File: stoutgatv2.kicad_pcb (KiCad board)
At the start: 2 copper layers, 345.7 x 99.5 mm, 191 parts, among them SW1 ESC, SW10 9, SW11 0, SW12 Rotary_Encoder_Switch, SW13 -, SW14 +, SW15 BKSPC, SW16 TILDE, SW17 TAB, SW18 Rotary_Encoder_Switch, SW19 Q, SW2 1, SW20 W, SW21 E, SW22 R, SW23 T, SW24 Y, SW25 U, SW26 I, SW27 O, SW28 P, SW29 [, SW3 2, SW30 ], SW31 ISO-ENTER, SW32 DEL, SW33 CAPS, SW34 A, SW35 S, SW36 D, SW37 F, SW38 G, SW39 H, SW4 3, SW40 J, SW41 K, SW42 L, SW43 ;, SW44 ', SW45 \, SW46 ANSISHIFT, SW47 CTRL-w, SW48 PGUP, SW49 SHIFT, SW5 4, SW50 <, SW51 Z, SW52 X, SW53 C, SW54 V, SW55 B, SW56 N, SW57 M, SW58 ,, SW59 ., SW6 5, SW60 /, SW61 SUPER-w, SW62 SHIFT, SW63 ^, SW64 PGDN, SW65 CTRL, SW66 SUPER, SW67 ALT, SW68 ALT-w, SW69 CTRL-w, SW7 6, SW70 ANSI-ENTER, SW71 SPACE, SW72 ANSI-|, SW73 CAPS, SW74 SPACE, SW75 ALT, SW76 FN, SW77 CTRL, SW78 <-, SW79 DN, SW8 7, SW80 ->, SW81 Rotary_Encoder_Switch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

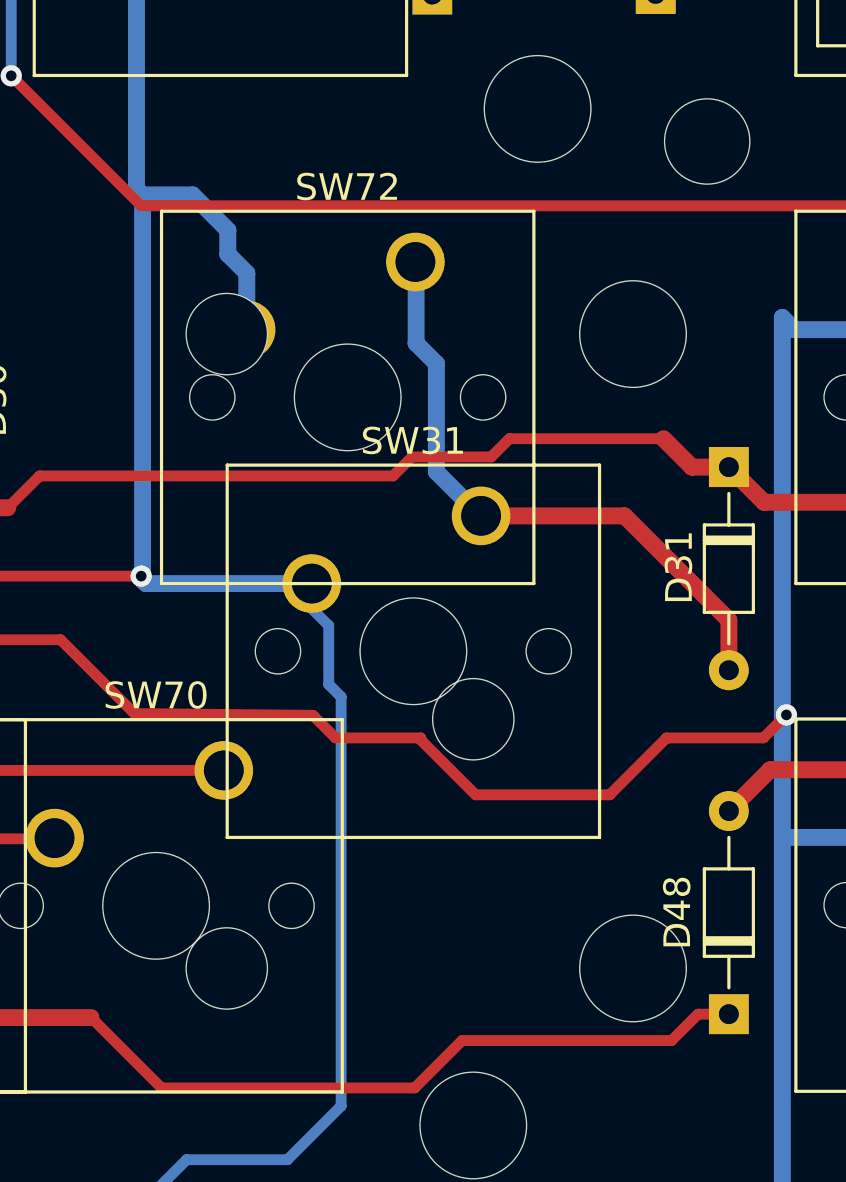
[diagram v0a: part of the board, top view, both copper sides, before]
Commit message: JLC tweaks
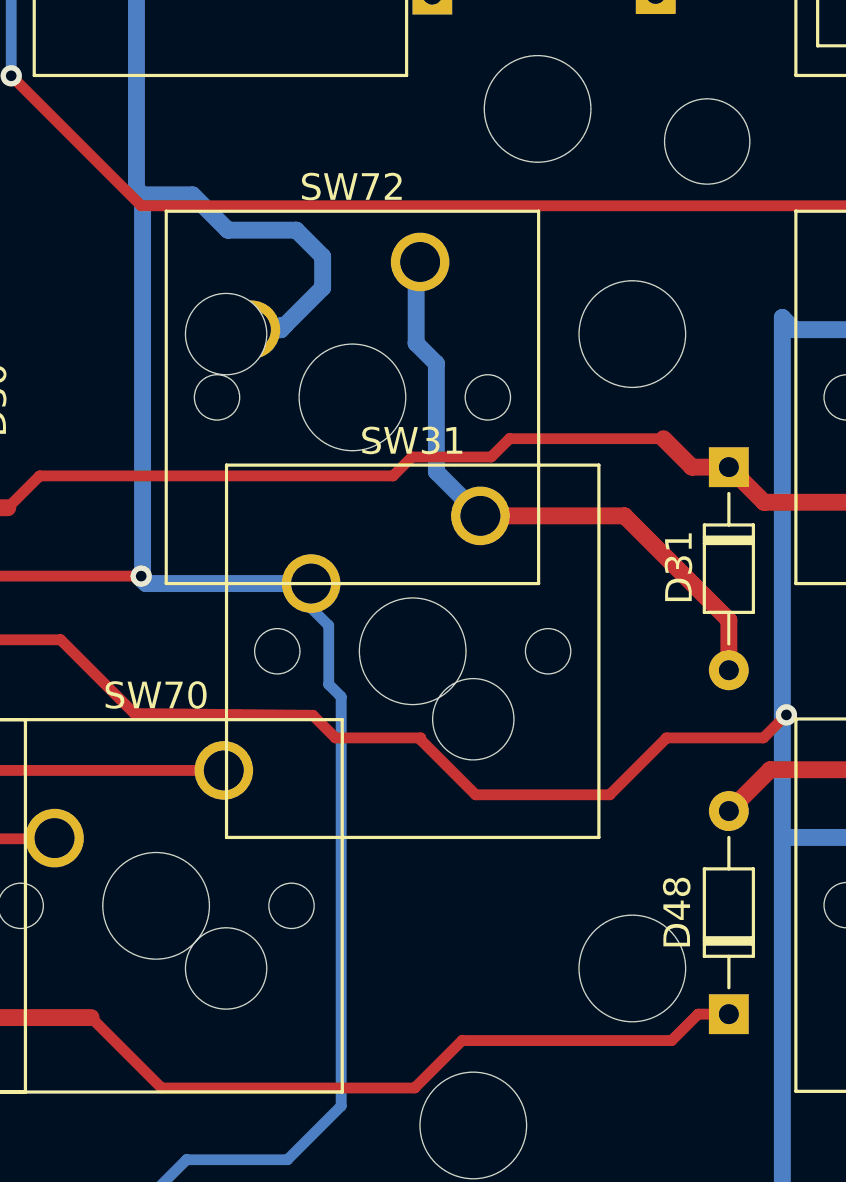
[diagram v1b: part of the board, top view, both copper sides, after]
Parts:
- moved SW72 0.18 mm to (354.5, 109.5)
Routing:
- net col13: track 422.9 -> 427.6 mm
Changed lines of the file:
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@@
     (thickness 1.6)
     (drawings 10)
-    (tracks 1026)
+    (tracks 1031)
     (zones 0)
     (modules 191)
@@
   )
   (setup
-    (last_trace_width 0.4064)
+    (last_trace_width 0.635)
     (user_trace_width 0.4064)
     (user_trace_width 0.635)
@@
     (visible_elements FFFDFF7F)
     (pcbplotparams
-      (layerselection 0x010fc_ffffffff)
+      (layerselection 0x01000_7ffffffe)
       (usegerberextensions false)
       (usegerberattributes false)
@@
       (psnegative false)
       (psa4output false)
-      (plotreference true)
-      (plotvalue true)
+      (plotreference false)
+      (plotvalue false)
       (plotinvisibletext false)
       (padsonsilk false)
       (subtractmaskfromsilk false)
-      (outputformat 1)
+      (outputformat 3)
       (mirror false)
-      (drillshape 0)
+      (drillshape 2)
       (scaleselection 1)
       (outputdirectory "gerbers/"))
@@
   )
   (module Button_Switch_Keyboard:SW_Cherry_MX_1.25u_PCB (layer F.Cu)
-    (at 354.33 109.4994)
+    (at 354.5078 109.4994)
     (descr "Cherry MX keyswitch, 1.25u, PCB mount, http://cherryamericas.com/wp-content/uploads/2014/12/mx_cat.pdf")
     (tags "Cherry MX keyswitch 1.25u PCB")
@@
   )
   (module Button_Switch_Keyboard:SW_Cherry_MX_ISOEnter_PCB locked (layer F.Cu)
-    (at 356.7938 119.0244)
+    (at 356.7684 119.0244)
     (descr "Cherry MX keyswitch, ISO Enter, PCB mount, http://cherryamericas.com/wp-content/uploads/2014/12/mx_cat.pdf")
     (tags "Cherry MX keyswitch ISO enter PCB")
@@
   (segment (start 347.2942 108.3056) (end 345.9734 106.9848) (width 0.635) (layer B.Cu) (net 97))
   (segment (start 345.9734 106.9848) (end 344.0938 106.9848) (width 0.635) (layer B.Cu) (net 97))
-  (segment (start 347.2942 109.20688) (end 347.2942 108.3056) (width 0.635) (layer B.Cu) (net 97))
-  (segment (start 348.0054 109.91808) (end 347.2942 109.20688) (width 0.635) (layer B.Cu) (net 97))
-  (segment (start 348.0054 112.0394) (end 348.0054 109.91808) (width 0.635) (layer B.Cu) (net 97))
   (segment (start 348.5896 163.569766) (end 348.5896 152.3238) (width 0.635) (layer B.Cu) (net 97))
   (segment (start 352.6536 150.1648) (end 349.377 150.1648) (width 0.4064) (layer B.Cu) (net 97))
@@
   (segment (start 345.6432 152.3238) (end 344.6272 151.3078) (width 0.4064) (layer B.Cu) (net 97))
   (segment (start 348.5896 152.3238) (end 345.6432 152.3238) (width 0.4064) (layer B.Cu) (net 97))
+  (segment (start 347.2942 108.3056) (end 349.8596 108.3056) (width 0.635) (layer B.Cu) (net 97))
+  (segment (start 349.8596 108.3056) (end 350.8502 109.2962) (width 0.635) (layer B.Cu) (net 97))
+  (segment (start 350.8502 110.4646) (end 349.4278 111.887) (width 0.635) (layer B.Cu) (net 97))
+  (segment (start 350.8502 109.2962) (end 350.8502 110.4646) (width 0.635) (layer B.Cu) (net 97))
+  (segment (start 349.296301 111.887) (end 349.296301 112.0394) (width 0.635) (layer B.Cu) (net 97))
+  (segment (start 349.4278 111.887) (end 349.296301 111.887) (width 0.635) (layer B.Cu) (net 97))
+  (segment (start 349.2754 112.0394) (end 349.4278 111.887) (width 0.635) (layer B.Cu) (net 97))
+  (segment (start 348.1578 112.0394) (end 349.2754 112.0394) (width 0.635) (layer B.Cu) (net 97))
   (segment (start 369.316 169.2148) (end 371.7798 169.2148) (width 0.635) (layer B.Cu) (net 98))
   (segment (start 368.0968 167.9956) (end 369.316 169.2148) (width 0.635) (layer B.Cu) (net 98))
